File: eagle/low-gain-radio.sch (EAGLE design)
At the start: 108 parts, among them Y1 32MHz

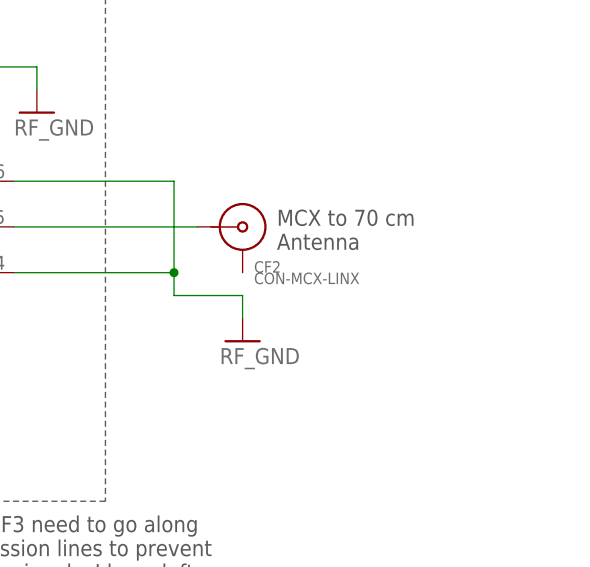
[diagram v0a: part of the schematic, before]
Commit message: Pushing for Andrew
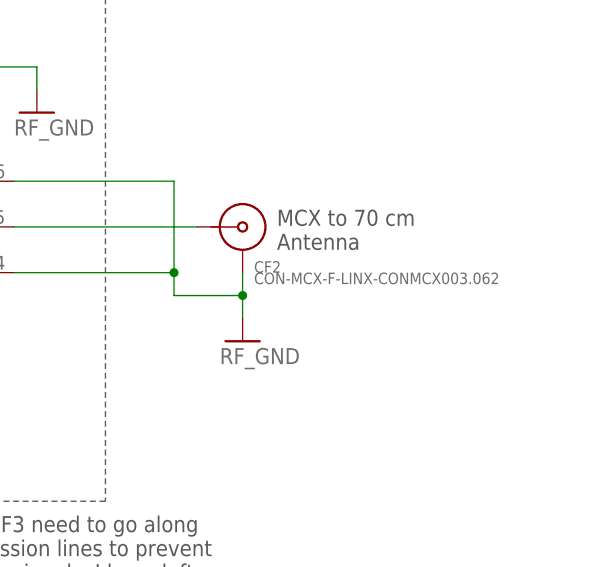
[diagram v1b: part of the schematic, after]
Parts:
- CF2: value CON-MCX-LINX -> CON-MCX-F-LINX-CONMCX003.062; device oresat-eagle:CON-MCX-LINX -> oresat-eagle:CON-MCX-F-LINX-CONMCX003.062
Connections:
- removed net ASD: C47.1
- net RF_GND: now also C47.1, CF2.SHIELD
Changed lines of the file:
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@@
 <part name="GND14" library="psas_c3_team05" deviceset="GND" device=""/>
 <part name="CF1" library="oresat-eagle" deviceset="ORESAT-CONNECTOR-40PIN" device=""/>
-<part name="CF2" library="oresat-eagle" deviceset="CON-MCX-LINX" device=""/>
+<part name="CF2" library="oresat-eagle" deviceset="CON-MCX-F-LINX-CONMCX003.062" device=""/>
 <part name="TP18" library="testpad" deviceset="TPS" device="PAD1-13"/>
 <part name="SH1" library="hw-laird-bmi-s-202" deviceset="BMI-S-202-SHIELD" device=""/>
@@
 </segment>
 </net>
-<net name="ASD" class="0">
-<segment>
-<pinref part="C47" gate="CE" pin="1"/>
-<wire x1="426.72" y1="175.26" x2="426.72" y2="172.72" width="0.1524" layer="91"/>
-<pinref part="U$38" gate="G$1" pin="GND"/>
-</segment>
-</net>
 <net name="N$2" class="0">
 <segment>
@@
 <wire x1="502.92" y1="167.64" x2="510.54" y2="167.64" width="0.1524" layer="91"/>
 <wire x1="510.54" y1="167.64" x2="510.54" y2="165.1" width="0.1524" layer="91"/>
+<pinref part="CF2" gate="G$1" pin="SHIELD"/>
+<wire x1="510.54" y1="170.18" x2="510.54" y2="167.64" width="0.1524" layer="91"/>
+<junction x="510.54" y="167.64"/>
 </segment>
 <segment>
@@
 <junction x="144.78" y="210.82"/>
 </segment>
-</net>
+<segment>
+<pinref part="C47" gate="CE" pin="1"/>
+<wire x1="426.72" y1="175.26" x2="426.72" y2="172.72" width="0.1524" layer="91"/>
+<pinref part="U$38" gate="G$1" pin="GND"/>
+</segment>
+</net>
